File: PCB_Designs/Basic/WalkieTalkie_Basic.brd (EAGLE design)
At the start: 33 x 50.8 mm, 60 parts, among them IC1 AD8609RU, IC2 AD8603UJ, IC3 MCP601OT, Q1 MOSFET-NCHANNELBSS123LT1G

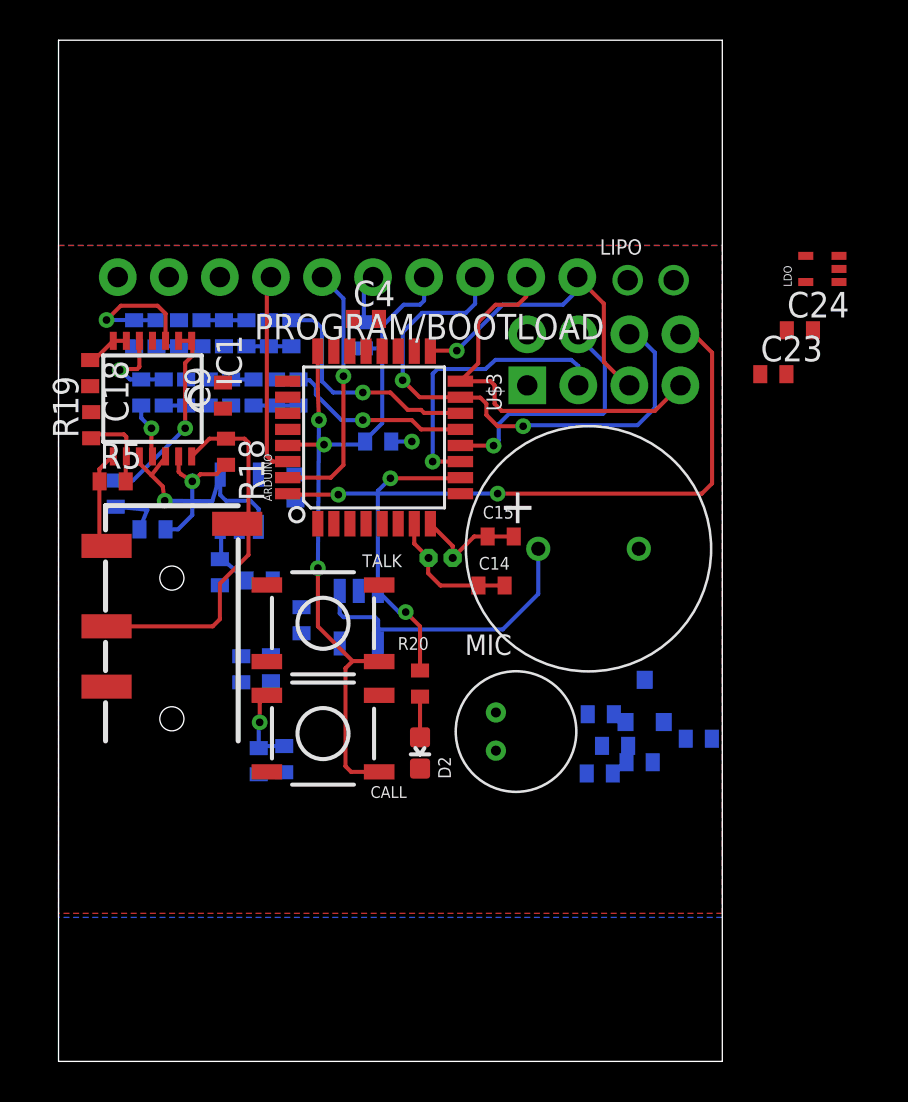
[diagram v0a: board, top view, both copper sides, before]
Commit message: more updates to PCB almost done
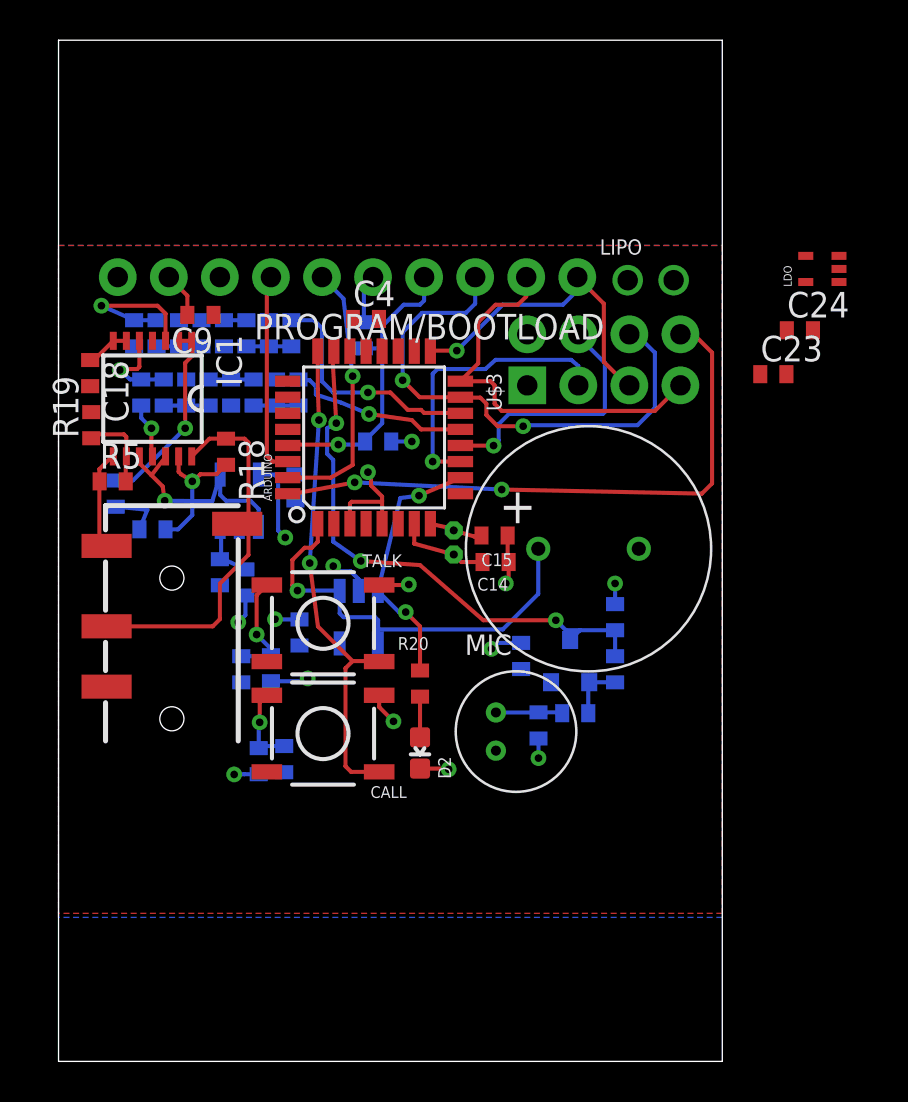
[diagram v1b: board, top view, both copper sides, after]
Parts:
- moved R2 7.34 mm to (27.7, 22.1), turned to 90 degrees
- moved R3 5.35 mm to (23.9, 16.7), turned to 270 degrees
- moved R1 5.24 mm to (27.7, 19.5), turned to 90 degrees
- moved C20 4.91 mm to (23.0, 20.2), turned to 270 degrees
- moved Q1 4.20 mm to (25.5, 19.9)
- moved C9 4.17 mm to (7.06, 37.1), turned to 180 degrees
- moved C1 2.56 mm to (25.7, 17.3), turned to 180 degrees
- moved XTAL 1.37 mm to (19.7, 26.4), turned to 270 degrees
- moved C14 1.19 mm to (21.7, 24.8), turned to 180 degrees
- moved R6 0.72 mm to (9.30, 23.8), turned to 90 degrees
- moved C22 0.62 mm to (12.0, 21.3)
- moved C15 0.31 mm to (21.7, 26.2), turned to 180 degrees
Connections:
- new net N$22: ARDUINO.25
- new net N$25: ARDUINO.26
- new net N$29: ARDUINO.27
- new net N$30: ARDUINO.28
- new net N$31: ARDUINO.19
- new net N$32: ARDUINO.22
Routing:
- net A0-MIC: track 0.00 -> 27.5 mm, vias 0 -> 3
- net 3.3V: track 1.03 -> 17.6 mm, vias 1 -> 10
- net GND: track 2.76 -> 17.5 mm, vias 1 -> 6
- net D3: track 15.3 -> 21.5 mm, vias 0 -> 1
- net N$2: track 0.00 -> 5.49 mm, vias 0 -> 1
- net N$8: track 0.00 -> 3.32 mm
- net N$21: track 5.64 -> 2.67 mm
- net N$5: track 0.00 -> 2.85 mm
- net N$20: track 6.82 -> 4.61 mm
- net D6: track 14.4 -> 13.0 mm
